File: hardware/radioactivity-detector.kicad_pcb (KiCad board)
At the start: 2 copper layers, 42.5 x 25 mm, 22 parts, among them J1 Conn_01x02, J2 Conn_01x02, U1 OPA333xxD, U2 OPA333xxD

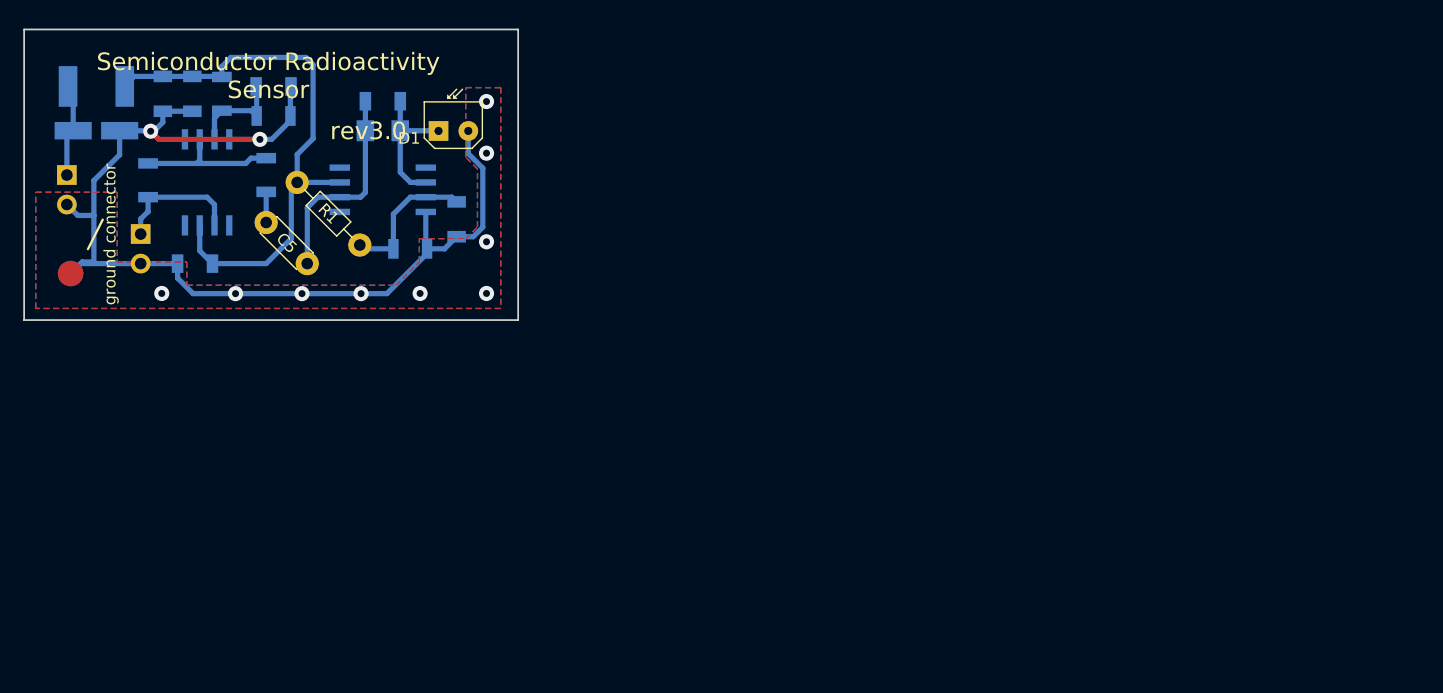
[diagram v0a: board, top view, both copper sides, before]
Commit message: initial versionwq
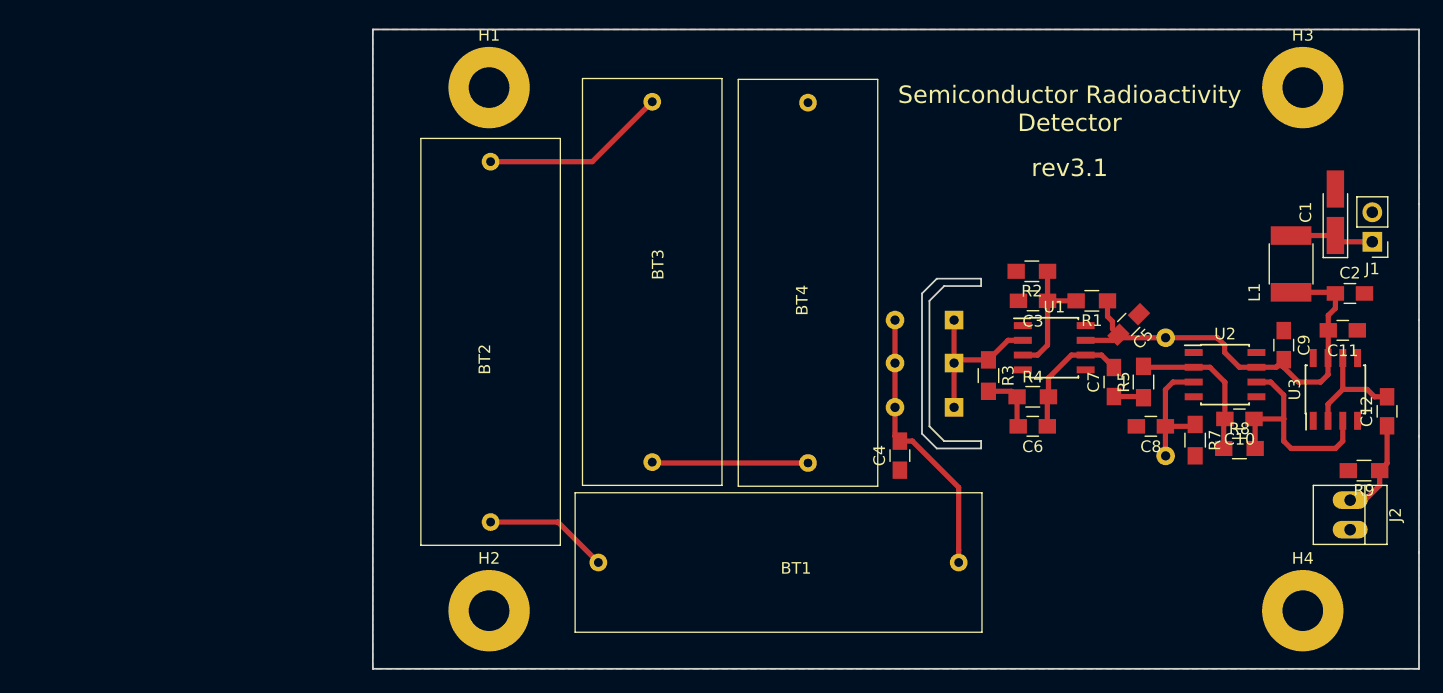
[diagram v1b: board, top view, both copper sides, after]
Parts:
- removed ground connector: MountingHole_2.2mm_M2, Mounting_Holes:MountingHole_2.2mm_M2
- added BT1: 12V, SemiconductorRadioactivityDetector:A23Single, F.Cu at (152.4, 109.9)
- added BT2: 12V, SemiconductorRadioactivityDetector:A23Single, F.Cu at (151.1, 79.4)
- added BT3: 12V, SemiconductorRadioactivityDetector:A23Single, F.Cu at (153.0, 109.2)
- added BT4: 12V, SemiconductorRadioactivityDetector:A23Single, F.Cu at (178.4, 74.3)
- added C10: 1p, Capacitors_SMD:C_0805_HandSoldering, F.Cu at (209.6, 103.5)
- added C11: 100n, Capacitors_SMD:C_0805_HandSoldering, F.Cu at (218.4, 95.9)
- added C12: 100n, Capacitors_SMD:C_0805_HandSoldering, F.Cu at (222.2, 102.8)
- added C9: 100n, Capacitors_SMD:C_0805_HandSoldering, F.Cu at (213.4, 97.2)
- added D2: D_Photo, Diodes_THT:D_DO-35_SOD27_P5.08mm_Vertical_KathodeUp, B.Cu at (185.0, 98.7)
- added D3: D_Photo, Diodes_THT:D_DO-35_SOD27_P5.08mm_Vertical_KathodeUp, B.Cu at (185.0, 95.0)
- added H1: MountingHole_Pad, Mounting_Holes:MountingHole_3.5mm_Pad, F.Cu at (145.0, 75.0)
- added H2: MountingHole_Pad, Mounting_Holes:MountingHole_3.5mm_Pad, F.Cu at (145.0, 120.0)
- added H3: MountingHole_Pad, Mounting_Holes:MountingHole_3.5mm_Pad, F.Cu at (215.0, 75.0)
- added H4: MountingHole_Pad, Mounting_Holes:MountingHole_3.5mm_Pad, F.Cu at (215.0, 120.0)
- added R8: 1M, Resistors_SMD:R_0805_HandSoldering, F.Cu at (209.6, 106.0)
- added R9: 10k, Resistors_SMD:R_0805_HandSoldering, F.Cu at (220.3, 108.0)
- added U3: OPA333xxD, Housings_SOIC:SOIC-8_3.9x4.9mm_Pitch1.27mm, F.Cu at (217.8, 101.0)
- C1: value 100n -> 100u; footprint Capacitors_SMD:C_1206 -> Capacitors_Tantalum_SMD:CP_Tantalum_Case-A_EIA-3216-18_Hand; moved to F.Cu
- C2, C4: footprint Capacitors_SMD:C_1206 -> Capacitors_SMD:C_0805_HandSoldering; moved to F.Cu
- C3: value 2p -> 100n; footprint Capacitors_SMD:C_1206 -> Capacitors_SMD:C_0805_HandSoldering; moved to F.Cu
- C5: value 1n -> 100n; footprint Capacitors_THT:C_Disc_D4.3mm_W1.9mm_P5.00mm -> Capacitors_SMD:C_0805_HandSoldering
- C6: value 100n -> 2p; footprint Capacitors_SMD:C_1206 -> Capacitors_SMD:C_0805_HandSoldering; moved to F.Cu
- C7: value 100n -> 1n; footprint Capacitors_SMD:C_1206 -> Capacitors_SMD:C_0805_HandSoldering; moved to F.Cu
- C8: value CP -> 100n; footprint Capacitors_Tantalum_SMD:CP_Tantalum_Case-A_EIA-3216-18_Hand -> Capacitors_SMD:C_0805_HandSoldering; moved to F.Cu
- D1: footprint Opto-Devices:PhotoDiode_BPW82 -> Diodes_THT:D_DO-35_SOD27_P5.08mm_Vertical_KathodeUp; moved to B.Cu
- J1: value Conn_01x02 -> power; footprint Pin_Headers:Pin_Header_Straight_2x01_Pitch2.54mm -> Connector_PinHeader_2.54mm:PinHeader_1x02_P2.54mm_Vertical; moved to F.Cu
- J2: value Conn_01x02 -> Conn_Coaxial; footprint Pin_Headers:Pin_Header_Straight_2x01_Pitch2.54mm -> Connectors:PINHEAD1-2; moved to F.Cu
- L1: moved to F.Cu
- R1: value 1k -> 10k; footprint Resistors_THT:R_Axial_DIN0204_L3.6mm_D1.6mm_P7.62mm_Horizontal -> Resistors_SMD:R_0805_HandSoldering
- R2, R7: value 1k -> 10k; footprint Resistors_SMD:R_1206 -> Resistors_SMD:R_0805_HandSoldering; moved to F.Cu
- R3: value 10M -> 560k; footprint Resistors_SMD:R_MiniMELF_MMA-0204 -> Resistors_SMD:R_0805_HandSoldering; moved to F.Cu
- R4: value 1k -> 560k; footprint Resistors_SMD:R_1206 -> Resistors_SMD:R_0805_HandSoldering; moved to F.Cu
- R5: footprint Resistors_SMD:R_1206 -> Resistors_SMD:R_0805_HandSoldering; moved to F.Cu
- R6: value 1M -> 10k; footprint Resistors_SMD:R_1206 -> Resistors_THT:R_Axial_DIN0207_L6.3mm_D2.5mm_P10.16mm_Horizontal
- U1, U2: footprint Housings_SOIC:SO-8_5.3x6.2mm_Pitch1.27mm -> Housings_SOIC:SOIC-8_3.9x4.9mm_Pitch1.27mm; moved to F.Cu
- moved J2 113.9 mm to (219.1, 110.5)
- moved J1 106.0 mm to (221.0, 88.3), turned to 180 degrees
- moved L1 103.9 mm to (214.0, 90.2), turned to 90 degrees
- moved C2 99.4 mm to (219.1, 92.7), turned to 0 degrees
- moved C8 94.2 mm to (201.9, 104.1), turned to 180 degrees
- moved U2 89.1 mm to (208.3, 99.7), turned to 0 degrees
- moved R6 88.6 mm to (203.2, 96.5)
- moved R7 84.0 mm to (205.7, 105.3), turned to 270 degrees
- moved C7 83.1 mm to (198.8, 100.3), turned to 90 degrees
- moved C6 80.1 mm to (191.8, 104.1), turned to 180 degrees
- moved R5 77.5 mm to (201.3, 100.3)
- moved C1 75.6 mm to (217.8, 85.7), turned to 90 degrees
- moved C5 74.7 mm to (200.0, 95.4), turned to 225 degrees
- moved R4 74.5 mm to (191.8, 101.6), turned to 0 degrees
- moved R1 69.1 mm to (196.8, 93.3), turned to 180 degrees
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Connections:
- C2 pad 1: Net-(C2-Pad1) -> Net-(C11-Pad2)
- C3 pad 2: Net-(C3-Pad2) -> GND
- C4 pad 1: Net-(C4-Pad1) -> GND
- C4 pad 2: GND -> Net-(BT1-Pad2)
- C5 pad 1: Net-(C5-Pad1) -> GND
- C5 pad 2: Net-(C3-Pad1) -> Net-(C11-Pad2)
- C6 pad 1: Net-(C2-Pad1) -> Net-(C6-Pad1)
- C6 pad 2: GND -> Net-(C6-Pad2)
- C7 pad 1: Net-(C2-Pad1) -> Net-(C7-Pad1)
- C7 pad 2: GND -> Net-(C6-Pad1)
- D1 pad 1: Net-(C3-Pad2) -> Net-(D1-Pad1)
- D1 pad 2: GND -> Net-(BT1-Pad2)
- J1 pad 1: Net-(J1-Pad1) -> Net-(C1-Pad1)
- J2 pad 1: Net-(C8-Pad1) -> Net-(C12-Pad1)
- L1 pad 1: Net-(C2-Pad1) -> Net-(C11-Pad2)
- L1 pad 2: Net-(C8-Pad1) -> Net-(C1-Pad1)
- R1 pad 1: Net-(C2-Pad1) -> Net-(C11-Pad2)
- R1 pad 2: Net-(C1-Pad1) -> Net-(C3-Pad1)
- R2 pad 1: Net-(C1-Pad1) -> Net-(C3-Pad1)
- R3 pad 1: Net-(C3-Pad2) -> Net-(D1-Pad1)
- R3 pad 2: Net-(C3-Pad1) -> Net-(C6-Pad2)
- R4 pad 1: Net-(C2-Pad1) -> Net-(C6-Pad2)
- R4 pad 2: Net-(C4-Pad1) -> Net-(C6-Pad1)
- R5 pad 1: Net-(C5-Pad1) -> Net-(C7-Pad1)
- R5 pad 2: Net-(R5-Pad2) -> Net-(C10-Pad2)
- R6 pad 1: Net-(R5-Pad2) -> Net-(C11-Pad2)
- R6 pad 2: Net-(J1-Pad1) -> Net-(C8-Pad1)
- R7 pad 1: Net-(C4-Pad1) -> Net-(C8-Pad1)
- U1 pad 2: Net-(C3-Pad2) -> Net-(D1-Pad1)
- U1 pad 3: Net-(C1-Pad1) -> Net-(C3-Pad1)
- U1 pad 6: Net-(C3-Pad1) -> Net-(C6-Pad1)
- U1 pad 7: Net-(C2-Pad1) -> Net-(C11-Pad2)
- U2 pad 2: Net-(R5-Pad2) -> Net-(C10-Pad2)
- U2 pad 3: Net-(C4-Pad1) -> Net-(C8-Pad1)
- U2 pad 6: Net-(J1-Pad1) -> Net-(C10-Pad1)
- U2 pad 7: Net-(C2-Pad1) -> Net-(C11-Pad2)
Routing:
- net GND: track 94.6 -> 0.00 mm, vias 11 -> 0
- net Net-(C2-Pad1): track 48.3 -> 0.00 mm
- net Net-(C11-Pad2): track 0.00 -> 38.7 mm
- net Net-(BT1-Pad2): track 0.00 -> 23.8 mm
- net Net-(C10-Pad1): track 0.00 -> 19.3 mm
- net Net-(BT2-Pad1): track 0.00 -> 16.0 mm
- net Net-(D1-Pad1): track 0.00 -> 14.2 mm
- net Net-(BT3-Pad1): track 0.00 -> 13.4 mm
- net Net-(C10-Pad2): track 0.00 -> 13.3 mm
- net Net-(R5-Pad2): track 12.5 -> 0.00 mm
- net Net-(C3-Pad2): track 12.3 -> 0.00 mm
- net Net-(J1-Pad1): track 11.2 -> 0.00 mm
- net Net-(C6-Pad1): track 0.00 -> 11.1 mm
- net Net-(BT1-Pad1): track 0.00 -> 10.7 mm
- net Net-(C12-Pad2): track 0.00 -> 10.00 mm
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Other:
- board size 42.5 x 25 mm -> 90 x 55 mm
- board text added: "Semiconductor Radioactivity Detector"
- board text added: "rev3.1"
- board text removed: "Semiconductor Radioactivity Sensor"
- board text removed: "rev3.0"
